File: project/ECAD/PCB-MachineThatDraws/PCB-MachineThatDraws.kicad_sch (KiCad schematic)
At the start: 15 parts, among them J1 SD_Card_Device, J2 SDA/SCL/VCC/GND, J3 Switch, J4 Switch, J5 Moteur, J6 Moteur, U1 ESP32-S3-UNO

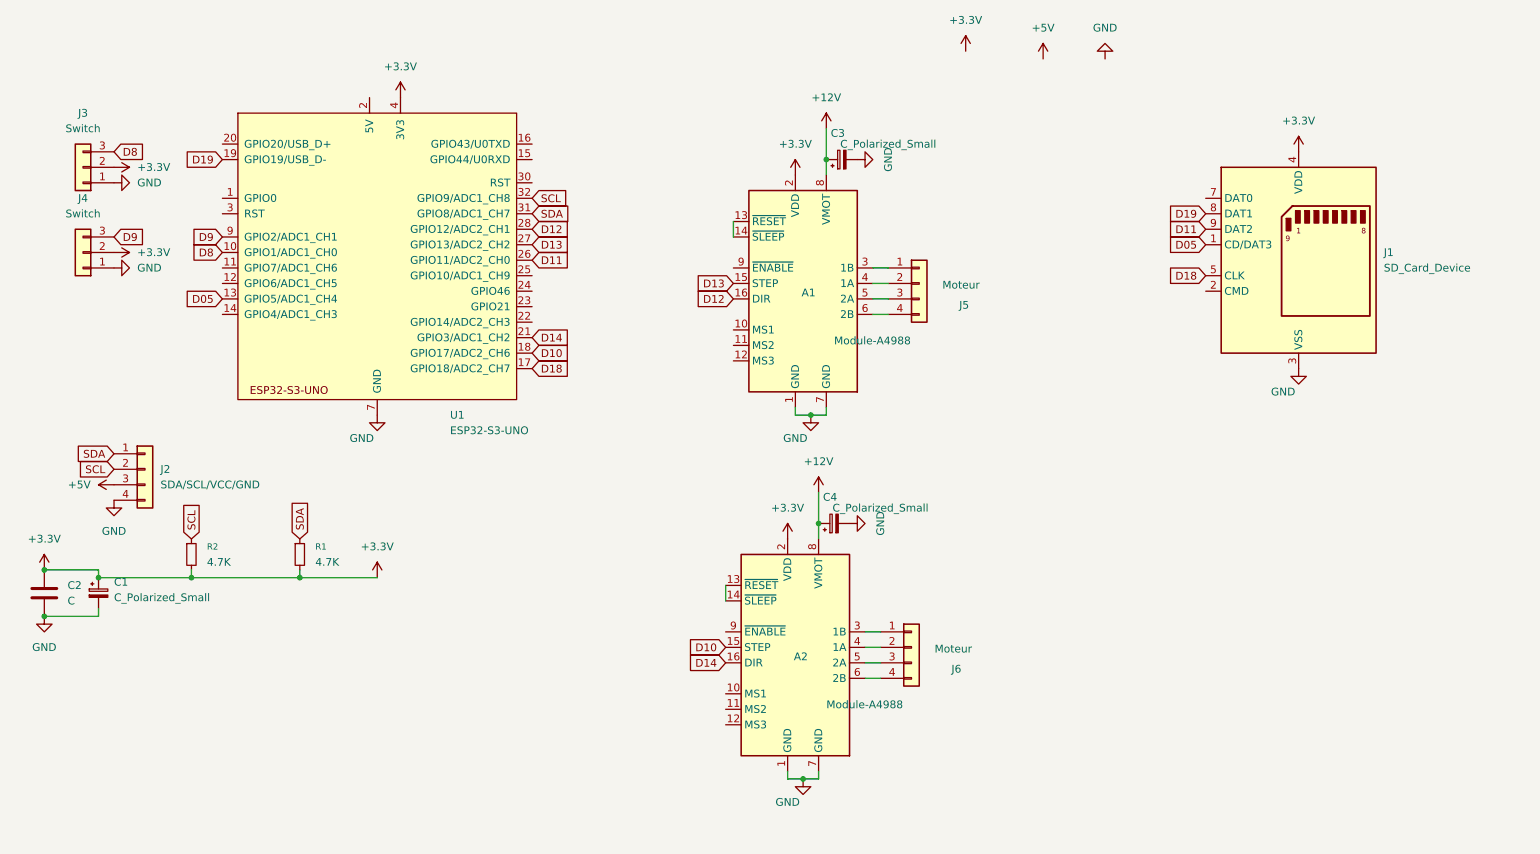
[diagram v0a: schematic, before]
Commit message: Update PCB-MachineThatDraws.kicad_sch
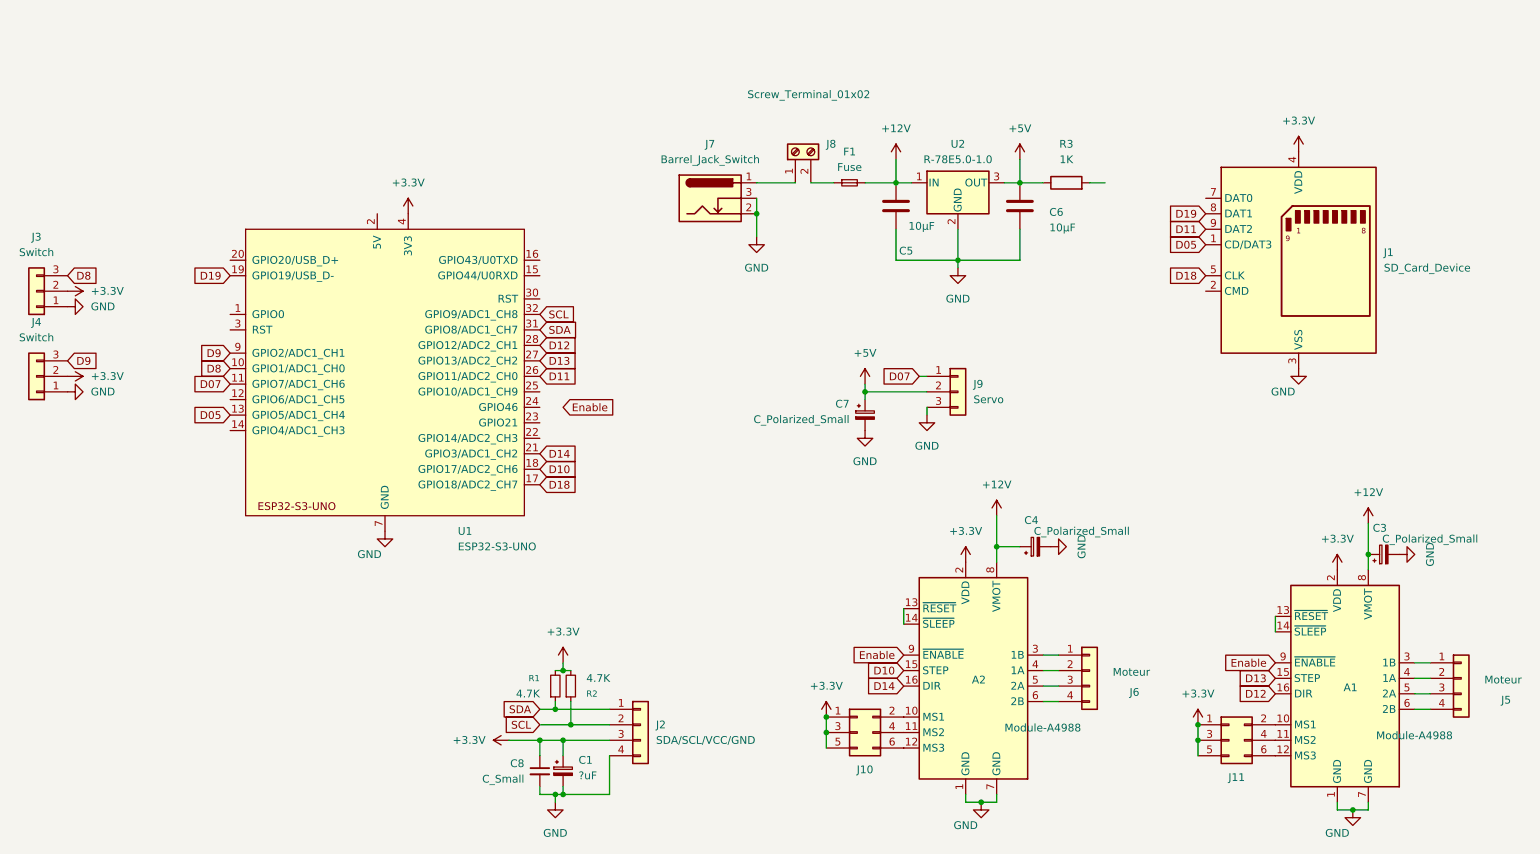
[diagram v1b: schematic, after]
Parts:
- removed C2: C, makerspace-unilasalle:C_1206, symbol Device:C
- added C5, C6: 10µF, symbol Device:C
- added C7: C_Polarized_Small, symbol Device:C_Polarized_Small
- added C8: C_Small, symbol Device:C_Small
- added F1: Fuse, symbol makerspace-unilasalle:Fuse
- added J10, J11: Conn_02x03_Odd_Even, Connector_PinHeader_2.54mm:PinHeader_2x03_P2.54mm_Vertical, symbol Connector_Generic:Conn_02x03_Odd_Even
- added J7: Barrel_Jack_Switch, symbol makerspace-unilasalle:Barrel_Jack_Switch
- added J8: Screw_Terminal_01x02, symbol makerspace-unilasalle:Screw_Terminal_01x02
- added J9: Servo, symbol makerspace-unilasalle:Conn_01x03
- added R3: 1K, symbol Device:R
- added U2: R-78E5.0-1.0, Converter_DCDC:Converter_DCDC_RECOM_R-78E-0.5_THT, symbol makerspace-unilasalle:R-78E5.0-1.0
- C1: value C_Polarized_Small -> ?uF
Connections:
- net +12V: now also C5.1, F1.2, U2.1 (IN)
- net +3.3V: now also J2.3 (Pin_3), C8.1, J10.1 (Pin_1), J10.3 (Pin_3), J10.5 (Pin_5), J11.1 (Pin_1), J11.3 (Pin_3), J11.5 (Pin_5)
- net +5V: now also C6.1, C7.1, J9.2 (Pin_2), R3.1, U2.3 (OUT); no longer J2.3 (Pin_3)
- net GND: now also C5.2, C6.2, C7.2, C8.2, J7.2, J7.3, J9.3 (Pin_3), U2.2 (GND)
- net SCL: no longer R2.1
- net SCL : now also R2.1
- net SDA: now also R1.1
- net SDA : no longer R1.1
- net at A1.10 (MS1): now also J11.2 (Pin_2)
- net at A1.11 (MS2): now also J11.4 (Pin_4)
- net at A1.12 (MS3): now also J11.6 (Pin_6)
- net Enable: now reaches A1.9 (~{ENABLE})
- net Enable: now also A2.9 (~{ENABLE})
- net D07: now reaches U1.11 (GPIO7/ADC1_CH6)
- net D07: now also J9.1 (Pin_1)
- net at A2.10 (MS1): now also J10.2 (Pin_2)
- net at A2.11 (MS2): now also J10.4 (Pin_4)
- net at A2.12 (MS3): now also J10.6 (Pin_6)
- new net: J7.1, J8.1 (Pin_1)
- new net: F1.1, J8.2 (Pin_2)
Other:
- moved on the sheet: A1, A2, C1, C3, C4, J2, J3, J4, J5, J6, R1, R2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
